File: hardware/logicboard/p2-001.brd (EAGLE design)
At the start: 72 x 72 mm, 53 parts, among them IC1 4066N, IC2 LTC485N, IC3 74LS07N, J1 LED, J2 PWR, J3 RLY, J4 Display, K1 G5V1, Q1 220mA/50V/3.5Ω, Q2 220mA/50V/3.5Ω, T1 2SC1815, U1 DS18B20

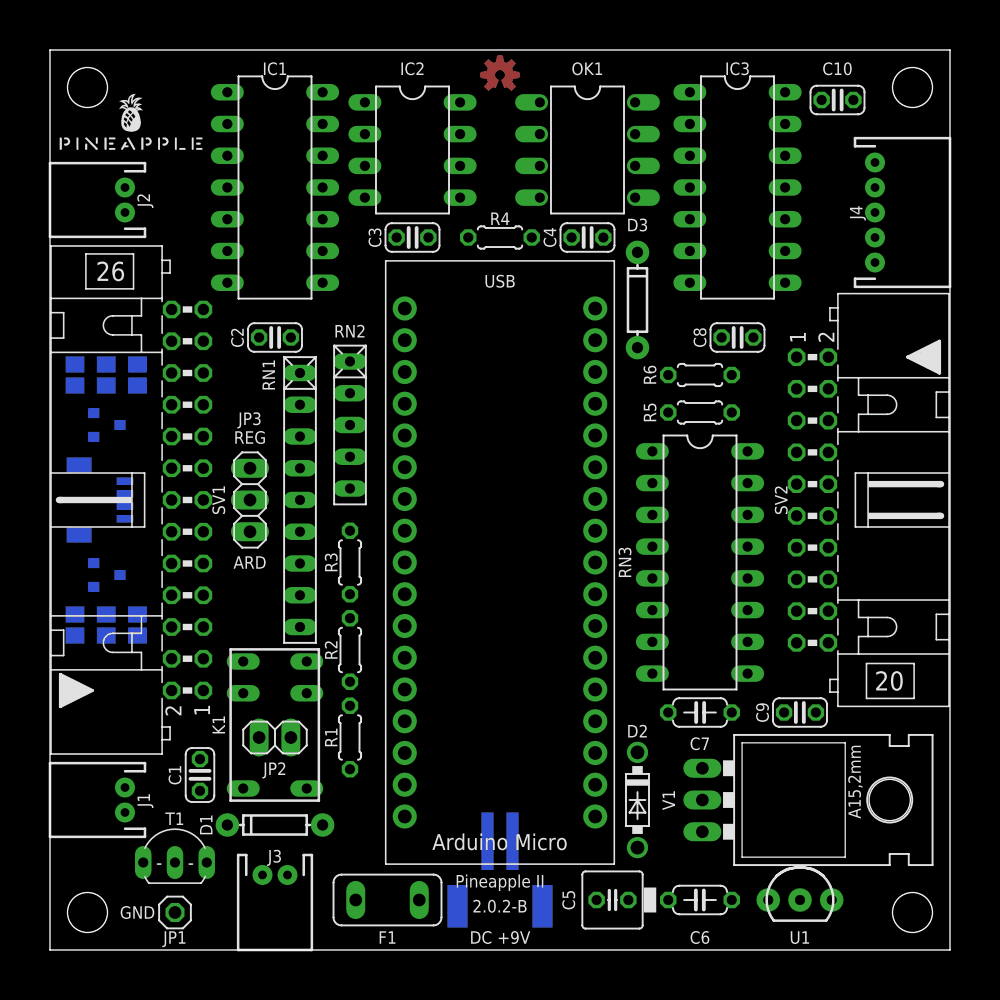
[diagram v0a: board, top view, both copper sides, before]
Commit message: Reflesh.
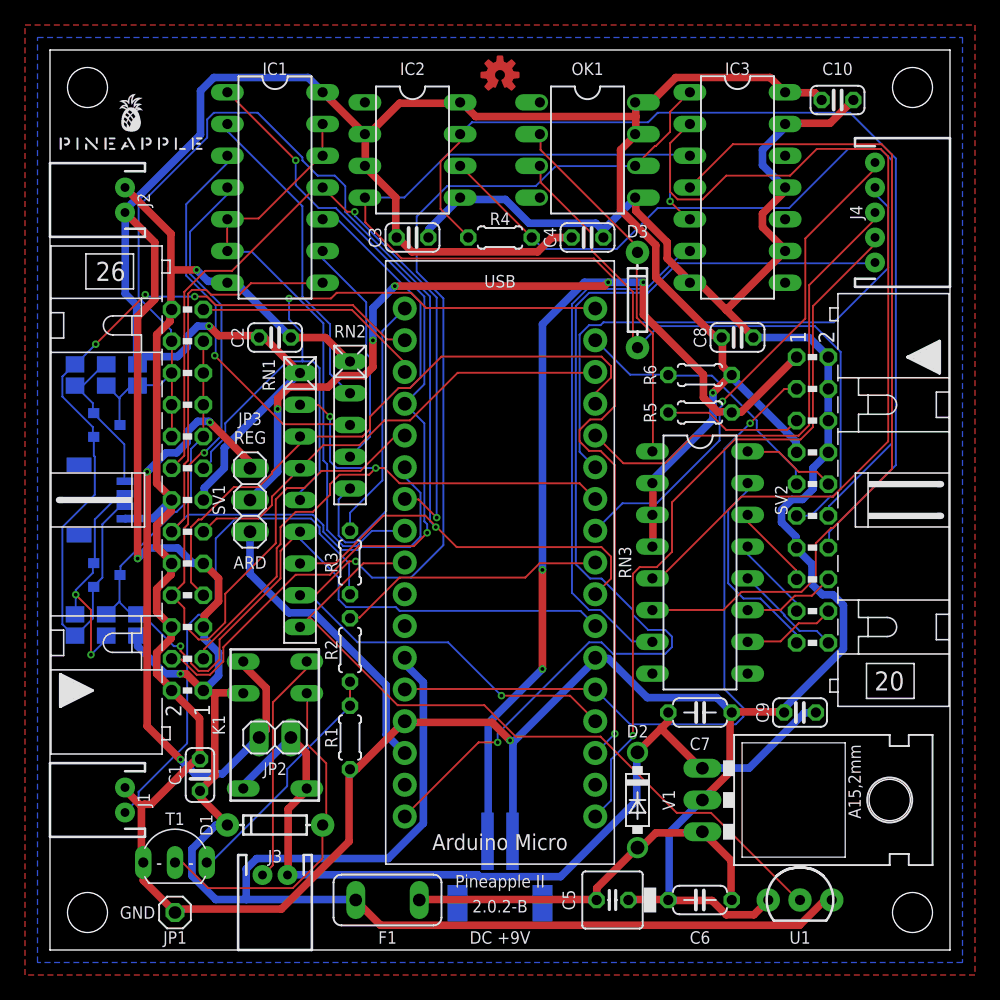
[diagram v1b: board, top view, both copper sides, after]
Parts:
- JP3: value (none) -> PWRSEL
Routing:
- net VCC: track 0.00 -> 347.1 mm, vias 0 -> 6
- net GND: track 0.00 -> 296.9 mm, vias 0 -> 2
- net +9V: track 0.00 -> 115.7 mm, vias 0 -> 7
- net SCL: track 0.00 -> 113.0 mm, vias 0 -> 1
- net TX: track 0.00 -> 99.2 mm, vias 0 -> 2
- net RX: track 0.00 -> 96.1 mm, vias 0 -> 2
- net SCLK: track 0.00 -> 85.4 mm, vias 0 -> 1
- net MTX-: track 0.00 -> 80.3 mm
- net SDA: track 0.00 -> 77.2 mm, vias 0 -> 1
- net V9A: track 0.00 -> 72.0 mm
- net MTH: track 0.00 -> 71.9 mm
- net MTX+: track 0.00 -> 71.6 mm
- net ANLG1: track 0.00 -> 70.3 mm, vias 0 -> 2
- net MO1: track 0.00 -> 68.6 mm
- net ANLG2: track 0.00 -> 67.7 mm, vias 0 -> 1
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- added copper zone on layer 1, net GND
- added copper zone on layer 16, net GND
